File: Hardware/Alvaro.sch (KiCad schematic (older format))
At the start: 26 parts, among them J2 01x02, J3 01x12, J4 01x12, J5 01x05, P1 USB_C_Receptacle_USB2.0, U1 ATmega32U4, X1 16MHz

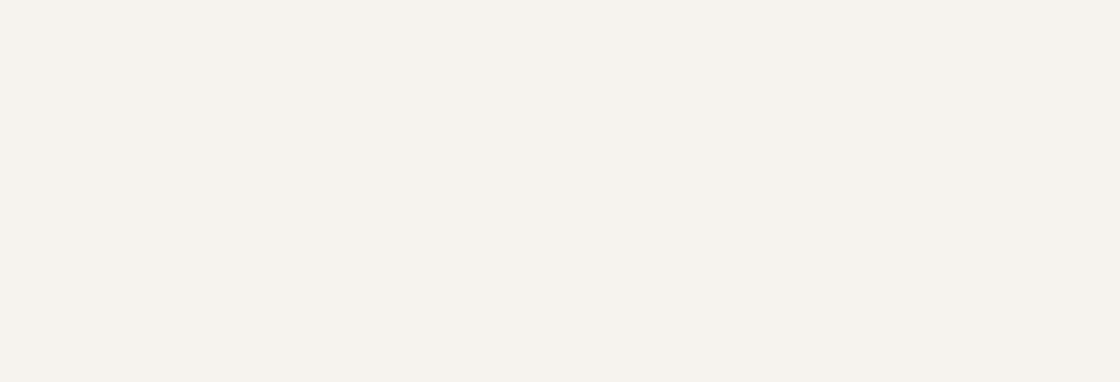
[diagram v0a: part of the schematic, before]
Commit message: Revert "Added THT pad under the 32u4."
This reverts commit 5261bc7efe342fde01f2eec8e41c6f0668064f92.
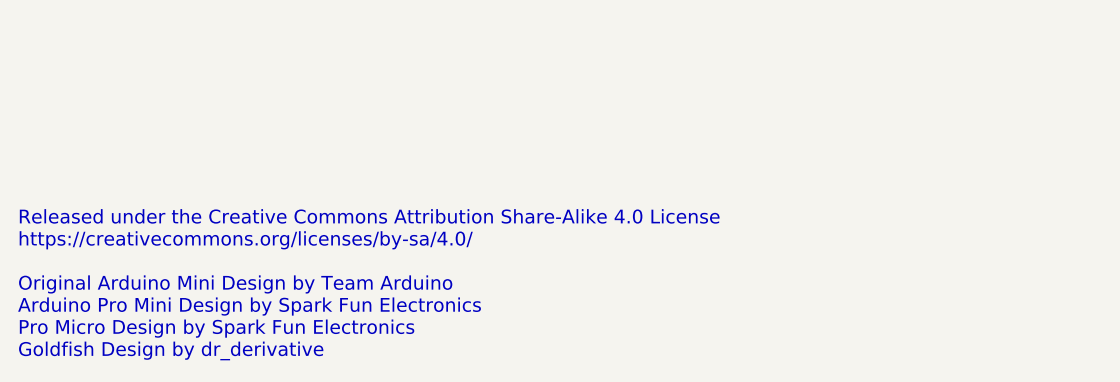
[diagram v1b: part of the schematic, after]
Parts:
- P1: footprint Alvaro:USB-C-C168688 -> Alvaro:USB-C_C168688
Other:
- note added: "Released under the Creative Commons Attribution Share-Alike 4.0 License\nhttps://creativecommons.org/licenses/by-sa/4.0/\n\nOriginal Arduino Mini Design by Team Arduino\nArduino Pro Mini Design by Spark Fun Electronics\nPro Micro Design by Spark Fun Electronics\nGoldfish Design by dr_derivative"
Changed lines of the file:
@@
 encoding utf-8
 Sheet 1 1
-Title "Alvaro"
-Date "2020-11-29"
-Rev "1.3"
+Title "Goldfish"
+Date "2017-12-20"
+Rev "C"
 Comp ""
 Comment1 ""
@@
 	5000 900  5000 800
 Connection ~ 5100 900
+Text Notes 700  7600 0    60   ~ 0
+Released under the Creative Commons Attribution Share-Alike 4.0 License\nhttps://creativecommons.org/licenses/by-sa/4.0/\n\nOriginal Arduino Mini Design by Team Arduino\nArduino Pro Mini Design by Spark Fun Electronics\nPro Micro Design by Spark Fun Electronics\nGoldfish Design by dr_derivative
 $Comp
 L power:VBUS #PWR016
@@
 F 0 "P1" H 2207 3067 50  0000 C CNN
 F 1 "USB_C_Receptacle_USB2.0" H 2207 2976 50  0000 C CNN
-F 2 "Alvaro:USB-C-C168688" H 2250 2200 50  0001 C CNN
+F 2 "Alvaro:USB-C_C168688" H 2250 2200 50  0001 C CNN
 F 3 "https://www.usb.org/sites/default/files/documents/usb_type-c.zip" H 2250 2200 50  0001 C CNN
 	1    2100 2200

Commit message: Added THT pad under the 32u4.
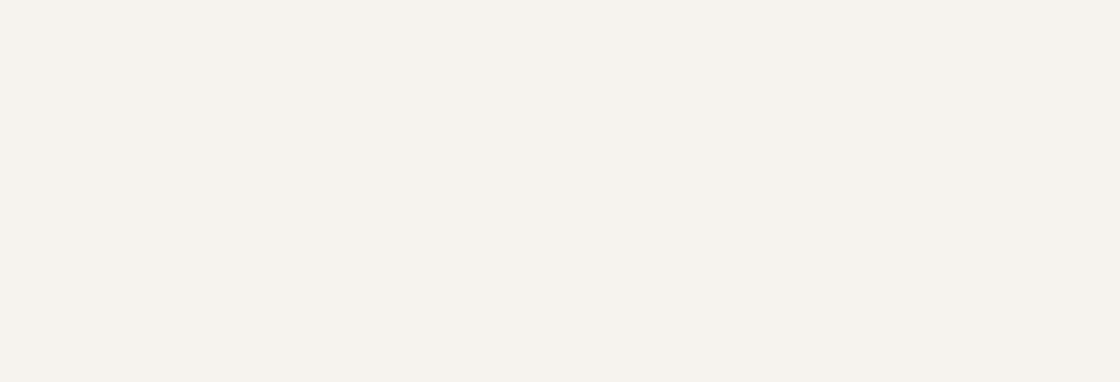
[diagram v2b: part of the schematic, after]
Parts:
- P1: footprint Alvaro:USB-C_C168688 -> Alvaro:USB-C-C168688
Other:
- note removed: "Released under the Creative Commons Attribution Share-Alike 4.0 License\nhttps://creativecommons.org/licenses/by-sa/4.0/\n\nOriginal Arduino Mini Design by Team Arduino\nArduino Pro Mini Design by Spark Fun Electronics\nPro Micro Design by Spark Fun Electronics\nGoldfish Design by dr_derivative"
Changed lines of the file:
@@
 encoding utf-8
 Sheet 1 1
-Title "Goldfish"
-Date "2017-12-20"
-Rev "C"
+Title "Alvaro"
+Date "2020-11-29"
+Rev "1.3"
 Comp ""
 Comment1 ""
@@
 	5000 900  5000 800
 Connection ~ 5100 900
-Text Notes 700  7600 0    60   ~ 0
-Released under the Creative Commons Attribution Share-Alike 4.0 License\nhttps://creativecommons.org/licenses/by-sa/4.0/\n\nOriginal Arduino Mini Design by Team Arduino\nArduino Pro Mini Design by Spark Fun Electronics\nPro Micro Design by Spark Fun Electronics\nGoldfish Design by dr_derivative
 $Comp
 L power:VBUS #PWR016
@@
 F 0 "P1" H 2207 3067 50  0000 C CNN
 F 1 "USB_C_Receptacle_USB2.0" H 2207 2976 50  0000 C CNN
-F 2 "Alvaro:USB-C_C168688" H 2250 2200 50  0001 C CNN
+F 2 "Alvaro:USB-C-C168688" H 2250 2200 50  0001 C CNN
 F 3 "https://www.usb.org/sites/default/files/documents/usb_type-c.zip" H 2250 2200 50  0001 C CNN
 	1    2100 2200
